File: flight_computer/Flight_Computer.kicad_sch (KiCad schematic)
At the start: 135 parts

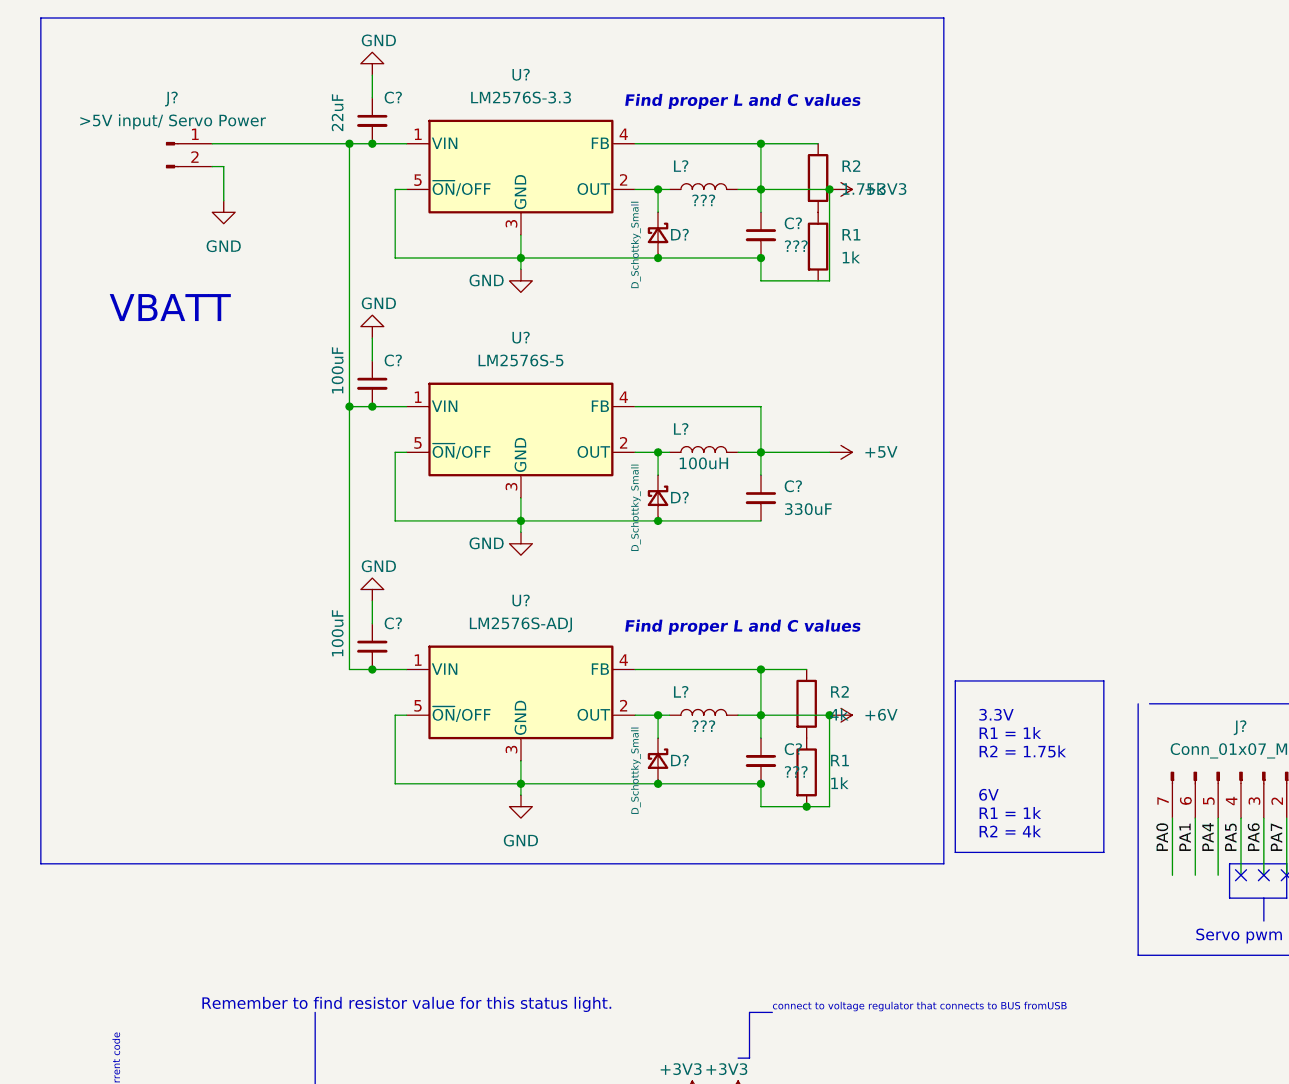
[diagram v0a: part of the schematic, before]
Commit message: ggg
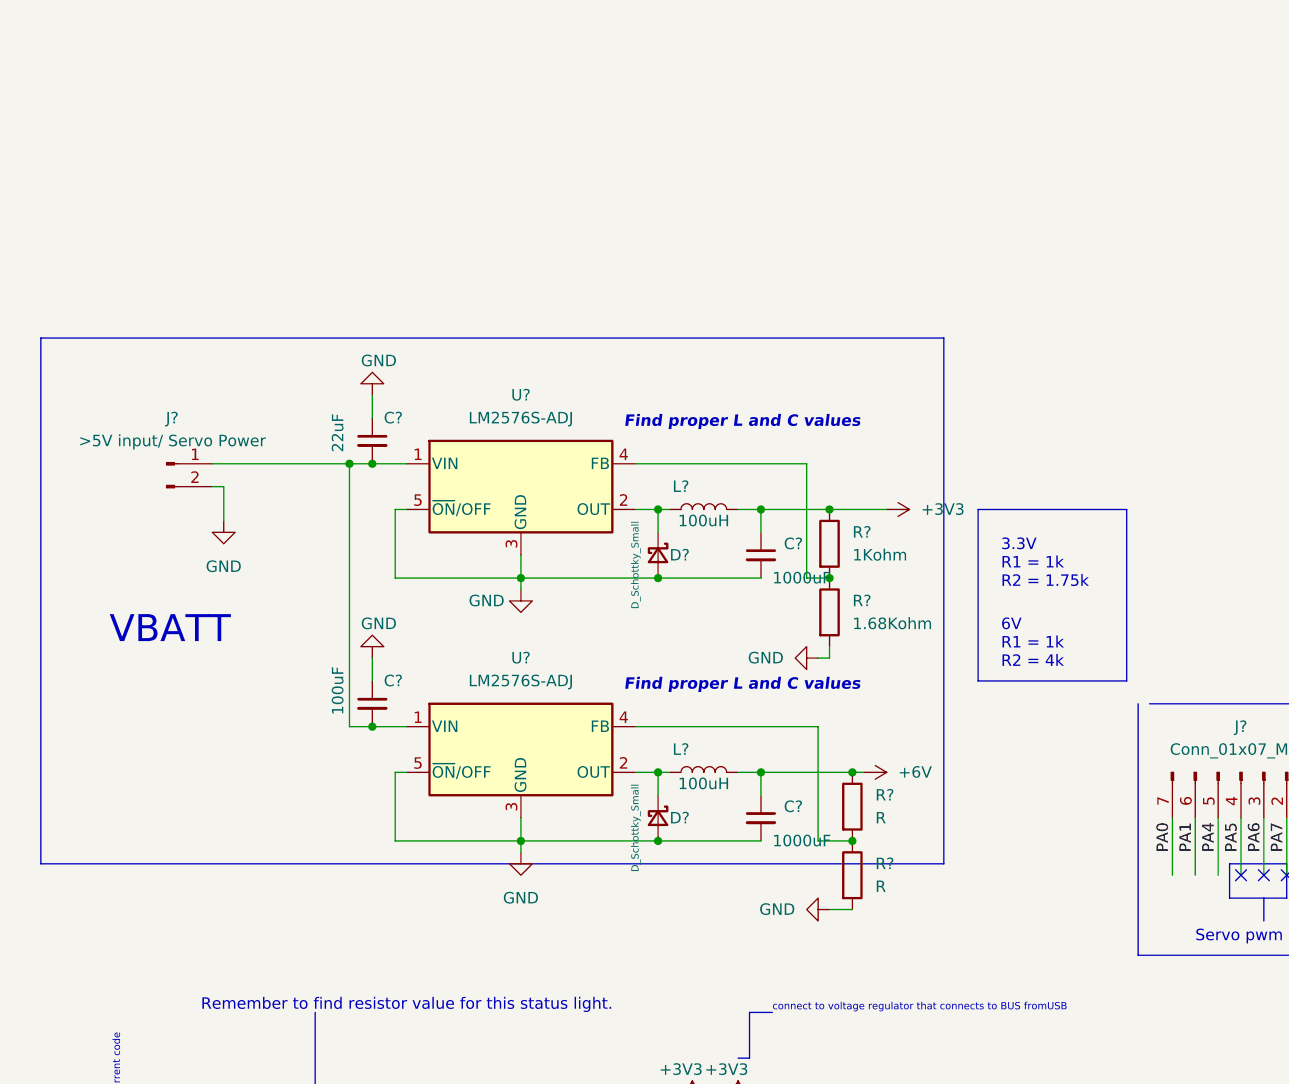
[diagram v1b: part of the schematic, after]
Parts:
- removed C?: ???, symbol Device:C_Small
- removed C?: 330uF, symbol Device:C_Small
- removed C?: 100uF, symbol Device:C_Small
- removed D?: D_Schottky_Small, symbol Device:D_Schottky_Small
- removed L?: ???, symbol Device:L
- removed L?: 100uH, symbol Device:L
- removed R1 (x2): 1k, symbol Device:R
- removed R2: 4k, symbol Device:R
- removed R2: 1.75k, symbol Device:R
- removed U?: LM2576S-5, Package_TO_SOT_SMD:TO-263-5_TabPin3, symbol Regulator_Switching:LM2576S-5
- removed U?: LM2576S-3.3, Package_TO_SOT_SMD:TO-263-5_TabPin3, symbol Regulator_Switching:LM2576S-3.3
- added C?: 1000uF, symbol Device:C_Small
- added L?: 100uH, symbol Device:L
- added R? (x2): R, symbol Device:R
- added R?: 1Kohm, symbol Device:R
- added R?: 1.68Kohm, symbol Device:R
- added U?: LM2576S-ADJ, Package_TO_SOT_SMD:TO-263-5_TabPin3, symbol Regulator_Switching:LM2576S-ADJ
- C?: value ??? -> 1000uF
- L?: value ??? -> 100uH
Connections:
- net +3V3: now also C?.1, L?.2, R?.1; no longer C?.1, C?.1, C?.1, C?.1, C?.1, C?.1, C?.1, C?.1, C?.1, C?.1, C?.1, C?.1, C?.1, C?.1, C?.1, C?.1, C?.2, C?.2, C?.2, C?.2, C?.2, C?.2, C?.2, C?.2, C?.2, C?.2, C?.2, C?.2, C?.2, C?.2, C?.2, C?.2, C?.2, C?.2, C?.2, C?.2, C?.2, C?.2, C?.2, C?.2, C?.2, C?.2, D?.2 (A), D?.2 (A), J?.1 (Pin_1), J?.1 (Pin_1), J?.1 (Pin_1), J?.2 (Pin_2), J?.4 (Pin_4), J?.6 (VSS), J?.A1 (GND), J?.A12 (GND), J?.A4 (VBUS), J?.A9 (VBUS), J?.B1 (GND), J?.B12 (GND), J?.B4 (VBUS), J?.B9 (VBUS), L?.2, L?.2, Male?.1 (Pin_1), Male?.1 (Pin_1), Q?.3 (S), Q?.3 (S), R?.1, R?.1, R?.1, R?.1, R?.1, R?.2, R?.2, R?.2, R?.2, R?.2, R?.2, R?.2, SW?.1 (A), U?.1 (GND), U?.15 (GNDIO), U?.16 (GNDIO), U?.18 (COM2), U?.2 (GND), U?.23 (VSS), U?.25 (GNDIO), U?.3 (GND), U?.3 (VI), U?.32 (EXT_XOSC), U?.33 (GND_EP), U?.35 (VSS), U?.4 (FB), U?.47 (VSS), U?.49 (VSS), U?.5 (~{ON}/OFF), U?.7 (GND), U?.8 (VSSA), U?.P$12 (GND@3), U?.P$19 (GND@4), U?.P$3 (GND@1), U?.P$8 (GND@2), VDiv1_?.1, VDiv2_?.1, X?.2, X?.4, Y?.2, Y?.4
- net at C?.2, C?.2, J?.1 (Pin_1)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: now also U?.1 (VIN)
- net at D?.1 (K): now also L?.1, U?.2 (OUT)
- new net: R?.1, R?.2, U?.4 (FB) (x2)
- new net +6V: C?.1, J?.1 (Pin_1), J?.1 (Pin_1), J?.1 (Pin_1), L?.2, R?.1
- new net GND: C?.1, C?.1, C?.1, C?.1, C?.1, C?.1, C?.1, C?.1, C?.1, C?.1, C?.1, C?.1, C?.1, C?.1, C?.1, C?.2, C?.2, C?.2, C?.2, C?.2, C?.2, C?.2, C?.2, C?.2, C?.2, C?.2, C?.2, C?.2, C?.2, C?.2, C?.2, C?.2, C?.2, C?.2, C?.2, C?.2, C?.2, C?.2, C?.2, C?.2, C?.2, C?.2, D?.2 (A), D?.2 (A), J?.2 (Pin_2), J?.4 (Pin_4), J?.6 (VSS), J?.A1 (GND), J?.A12 (GND), J?.A4 (VBUS), J?.A9 (VBUS), J?.B1 (GND), J?.B12 (GND), J?.B4 (VBUS), J?.B9 (VBUS), L?.2, Male?.1 (Pin_1), Male?.1 (Pin_1), Q?.3 (S), Q?.3 (S), R?.1, R?.1, R?.1, R?.1, R?.1, R?.2, R?.2, R?.2, R?.2, R?.2, R?.2, R?.2, R?.2, R?.2, SW?.1 (A), U?.1 (GND), U?.15 (GNDIO), U?.16 (GNDIO), U?.18 (COM2), U?.2 (GND), U?.23 (VSS), U?.25 (GNDIO), U?.3 (GND), U?.3 (GND), U?.3 (VI), U?.32 (EXT_XOSC), U?.33 (GND_EP), U?.35 (VSS), U?.47 (VSS), U?.49 (VSS), U?.5 (~{ON}/OFF), U?.5 (~{ON}/OFF), U?.7 (GND), U?.8 (VSSA), U?.P$12 (GND@3), U?.P$19 (GND@4), U?.P$3 (GND@1), U?.P$8 (GND@2), VDiv1_?.1, VDiv2_?.1, X?.2, X?.4, Y?.2, Y?.4
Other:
- moved on the sheet: C?, D?, J?, L?, U?
